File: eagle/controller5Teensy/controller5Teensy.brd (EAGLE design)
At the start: 53.3 x 64.8 mm, 63 parts, among them Q1 MMBT4403, U1 LM75AIM, U3 mp2307, U4 ATSAMD21G-A, X2 ZX62D-B-5PA8

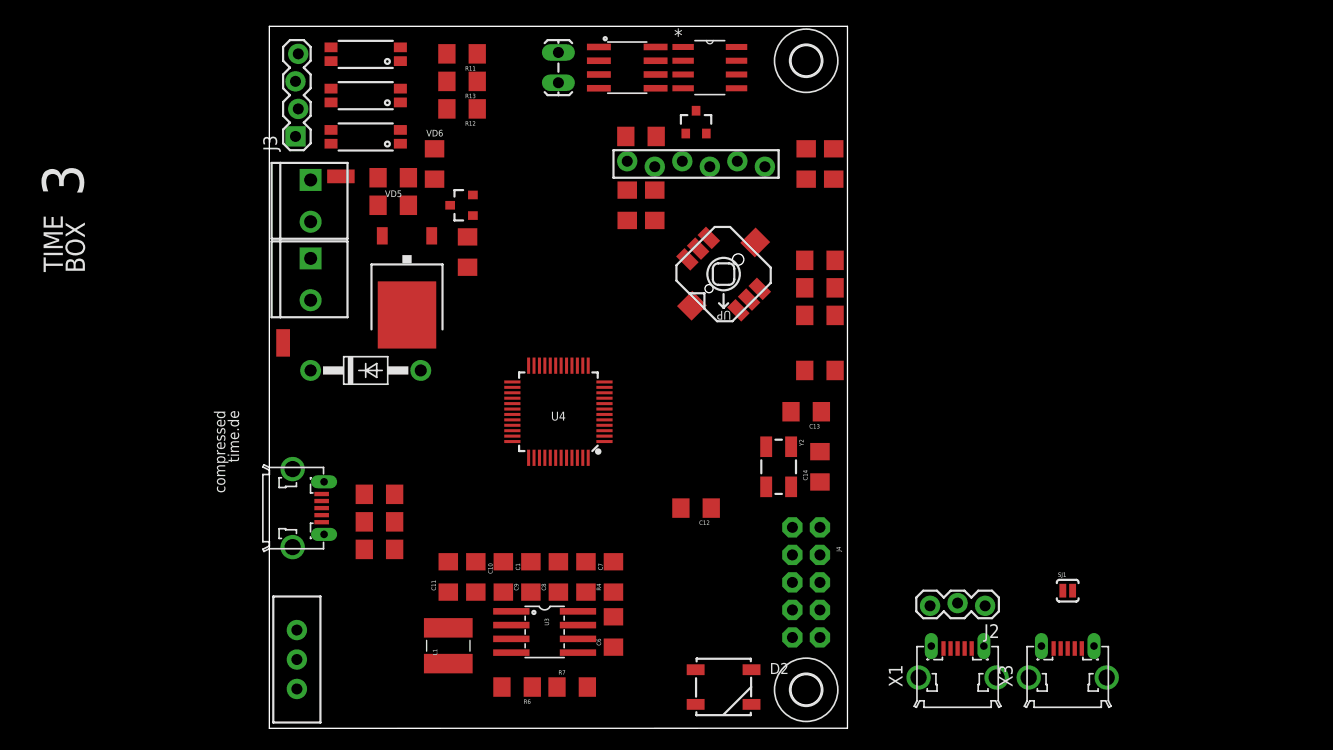
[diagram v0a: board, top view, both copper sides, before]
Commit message: controller5 & controller5Teensy
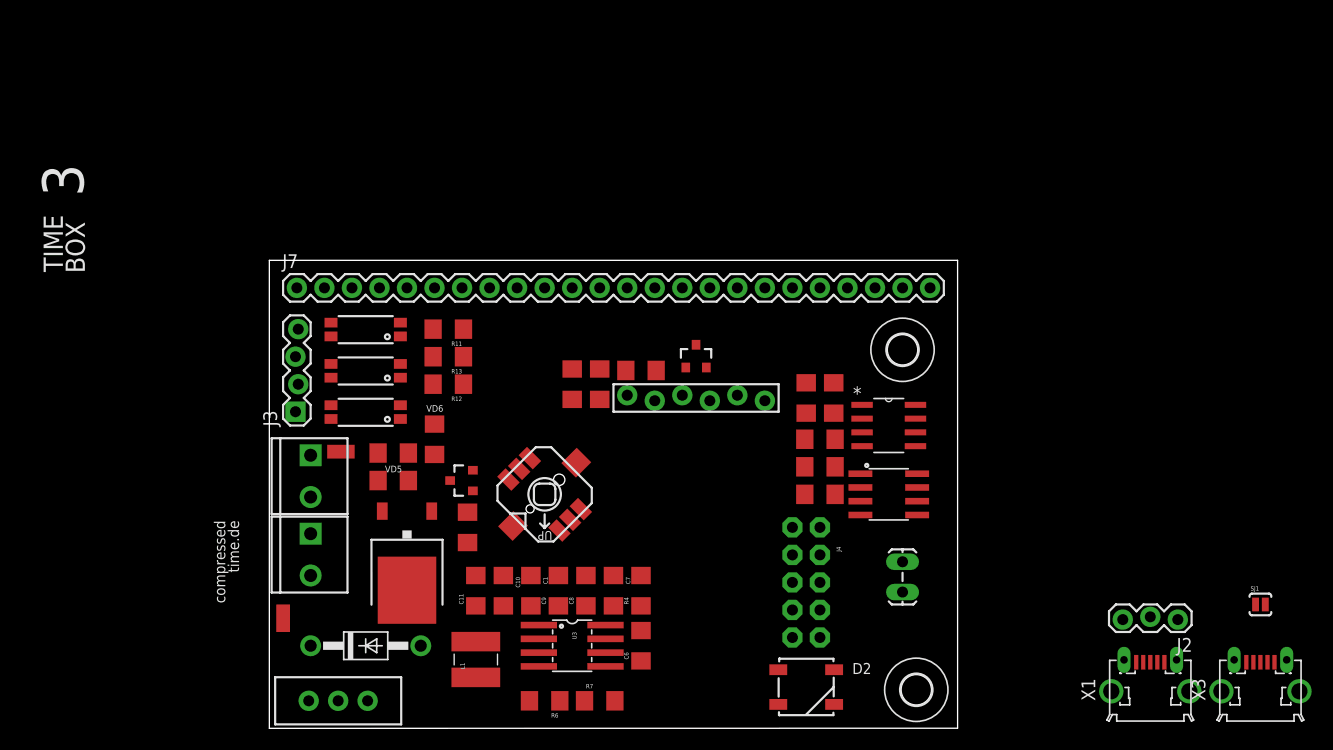
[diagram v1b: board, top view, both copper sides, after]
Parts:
- removed C12: 1uF, SparkFun-Capacitors:1206
- removed C13, C14: 22pF, SparkFun-Passives:1206
- removed C3: 10uF, SparkFun-Passives:1206
- removed RRST, RUSB1, RUSB2: (no value), SparkFun-Passives:1206
- removed U4: ATSAMD21G-A, SparkFun-DigitalIC:TQFP-48
- removed X2: ZX62D-B-5PA8, zx62d-b-5pa8-oshpark_10:ZX62D-B-5PA8
- removed Y2: (no value), SparkFun-FreqCtrl:CRYSTAL-SMD-5X3
- added J7: (no value), SparkFun-Connectors:1X24
- moved J1 56.7 mm to (58.4, 15.2)
- moved RTC1 46.2 mm to (57.1, 21.6)
- moved U1 36.9 mm to (57.1, 27.9)
- moved H3 28.1 mm to (58.4, 34.9)
- moved S1 26.2 mm to (25.4, 21.6)
- moved R11 25.4 mm to (16.5, 36.8)
- moved R12 25.4 mm to (16.5, 31.8)
- moved R13 25.4 mm to (16.5, 34.3)
- moved D1 25.4 mm to (8.89, 7.62)
- moved SH1 25.4 mm to (1.27, 10.2)
- moved J3 25.4 mm to (2.54, 29.2)
- moved J5 25.4 mm to (3.81, 25.0)
- moved J6 25.4 mm to (3.81, 17.8)
- moved Q2 25.4 mm to (12.7, 15.2)
- moved R17 25.4 mm to (11.4, 22.9)
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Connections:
- removed net D+: RUSB2.1, U4.34
- removed net D-: RUSB1.1, U4.33
- removed net MISO: U4.21
- removed net MOSI: U4.19
- removed net N$10: RUSB1.2, X2.2
- removed net N$11: RUSB2.2, X2.3
- removed net N$2: U4.45
- removed net N$25: C12.2, U4.43
- removed net N$27: C13.2, U4.1, Y2.3
- removed net N$28: C14.2, U4.2, Y2.1
- removed net N$3: U4.46
- removed net RST: RRST.1, U4.40
- removed net RX: U4.38
- removed net SCK: U4.20
- removed net TX: U4.37
- net GND: no longer C12.1, C13.1, C14.1, C3.2, U4.18, U4.35, U4.42, U4.5, X2.5
- net N$22: no longer C3.1, X2.1
- net SCL: no longer U4.32
- net SDA: no longer U4.31
- net VCC: no longer RRST.2, U4.17, U4.36, U4.44, U4.6
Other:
- board size 53.3 x 64.8 mm -> 63.5 x 43.2 mm
